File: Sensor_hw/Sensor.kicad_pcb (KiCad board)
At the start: 2 copper layers, 29 x 32.5 mm, 18 parts, among them Q1 TSOP48xx, Q2 TSOP48xx, Q3 TSOP48xx, Q4 WS2812B

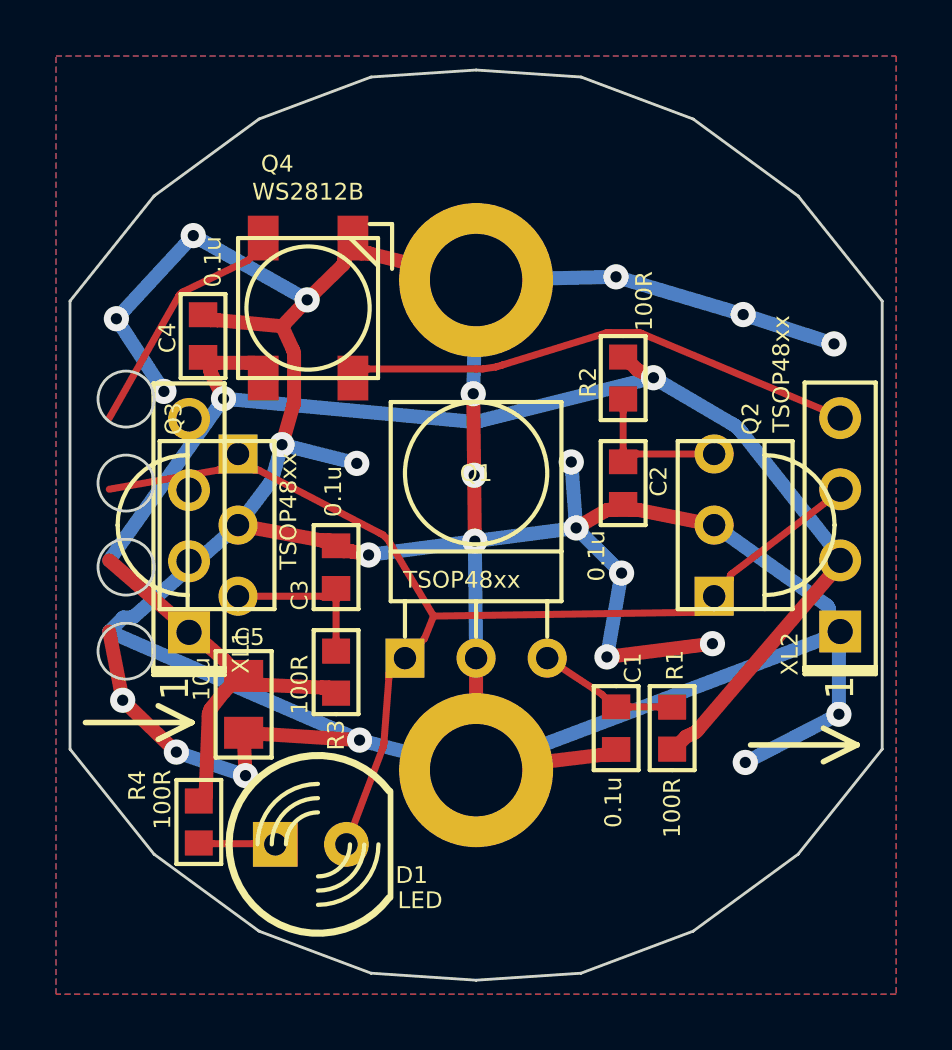
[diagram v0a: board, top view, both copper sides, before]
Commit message: + Sensor sent to manufacture * Head: barrel socket is here + armlet case
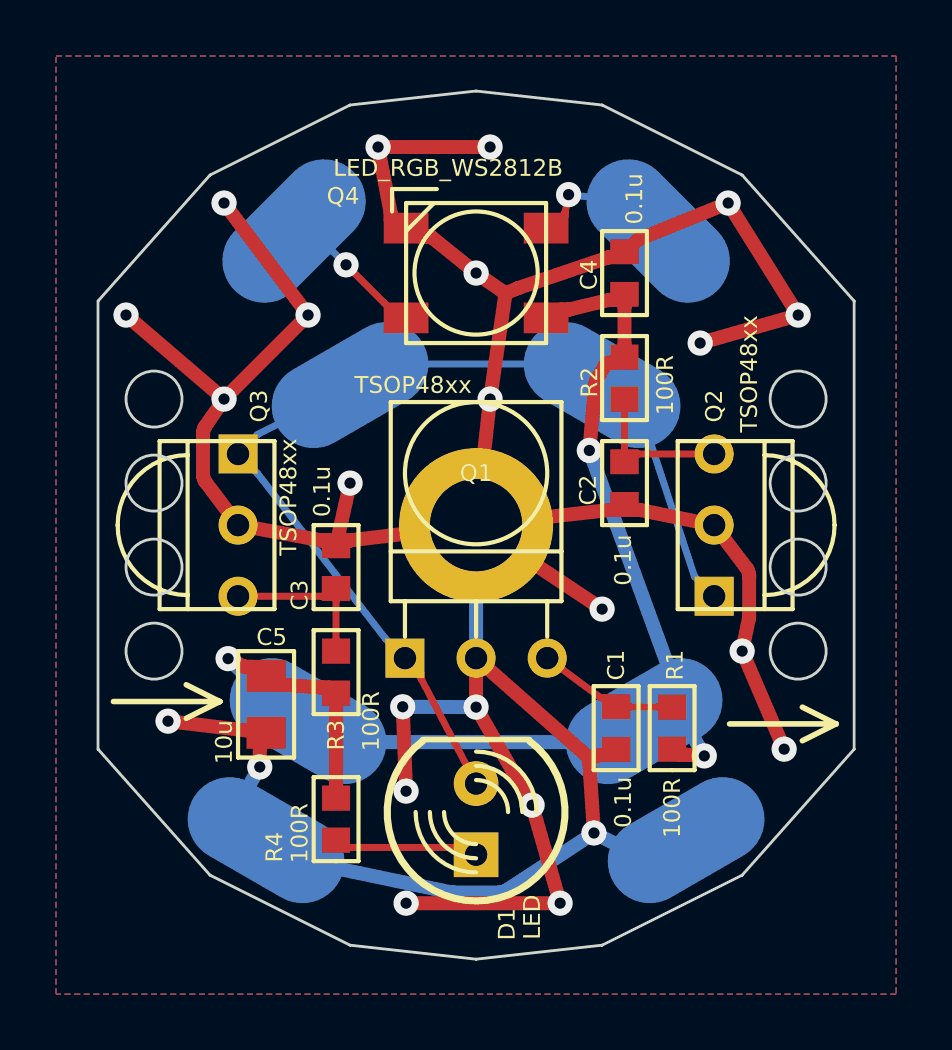
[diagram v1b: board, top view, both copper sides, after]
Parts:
- removed HOLE2: HOLE_METALLED, PCB:Hole3d3_out5d5mm
- added XL3: CONN_1, PCB:Oval6x3, B.Cu at (144.0, 100.0)
- added XL4: CONN_1, PCB:Oval6x3, B.Cu at (142.0, 94.5)
- added XL5: CONN_1, PCB:Oval6x3, B.Cu at (156.0, 116.2)
- added XL6: CONN_1, PCB:Oval6x3, B.Cu at (154.5, 112.0)
- added XL7: CONN_1, PCB:Oval6x3, B.Cu at (153.0, 100.0)
- added XL8: CONN_1, PCB:Oval6x3, B.Cu at (155.0, 94.5)
- Q4: value WS2812B -> LED_RGB_WS2812B
- XL1, XL2: value CONN_4 -> CONN_1; footprint Connectors:PLS-4 -> PCB:Oval6x3; moved to B.Cu
- moved XL2 19.3 mm to (142.5, 112.0), turned to 330 degrees
- moved C4 15.2 mm to (153.8, 96.0)
- moved HOLE1 8.75 mm to (148.5, 105.0)
- moved XL1 7.91 mm to (141.0, 116.2), turned to 150 degrees
- moved Q4 6.13 mm to (148.5, 96.0), turned to 180 degrees
- moved D1 5.97 mm to (148.5, 115.5), turned to 90 degrees
- moved R4 4.90 mm to (143.5, 115.5)
- moved C5 0.80 mm to (141.0, 111.4)
- moved C2 0.05 mm to (153.8, 103.5)
- moved R2 0.05 mm to (153.8, 99.8)
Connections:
- XL2 pad 1: GND -> VCC
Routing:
- net /LED_DOUT: track 18.4 -> 5.24 mm, vias 0 -> 1
- net VCC: track 61.8 -> 48.8 mm, vias 2 -> 3
- net GND: track 159.4 -> 149.1 mm
- net /LED_DIN: track 8.78 -> 5.50 mm, vias 0 -> 1
- net Net-(D1-PadA): track 2.73 -> 5.13 mm
- net /SNS: track 39.6 -> 37.7 mm
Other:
- board size 29 x 32.5 mm -> 27 x 31 mm
- rule pad_to_mask_clearance: 0.2 -> 0.1
- board text added: "GND"
- board text added: "LED DIN"
- board text added: "LED DOUT"
- board text added: "SNS"
- board text added: "VCC"
